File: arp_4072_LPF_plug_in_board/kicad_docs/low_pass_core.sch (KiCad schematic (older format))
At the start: 46 parts, among them Q1 BCM857DS, Q2 BCM857DS, Q3 BCM857DS, Q4 BCM857DS, Q5 BCM857DS, Q6 BCM857DS, U1 LM3900, U2 TL072, U3 TL072

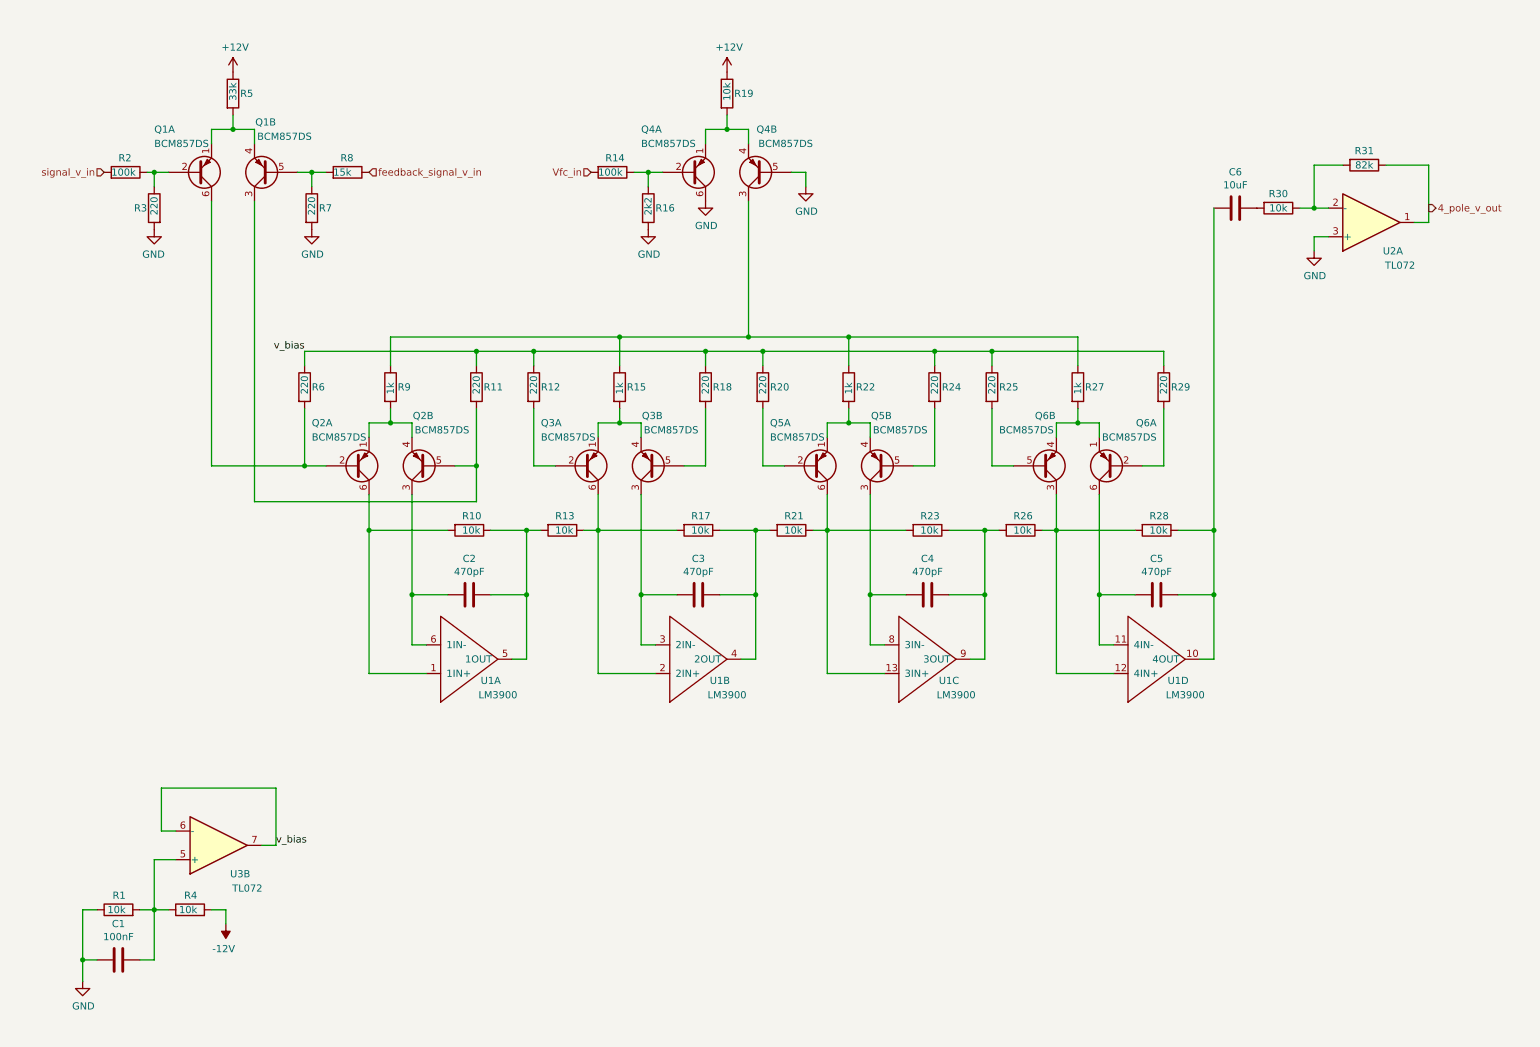
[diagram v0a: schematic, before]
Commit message: fix schemo and pcb problems
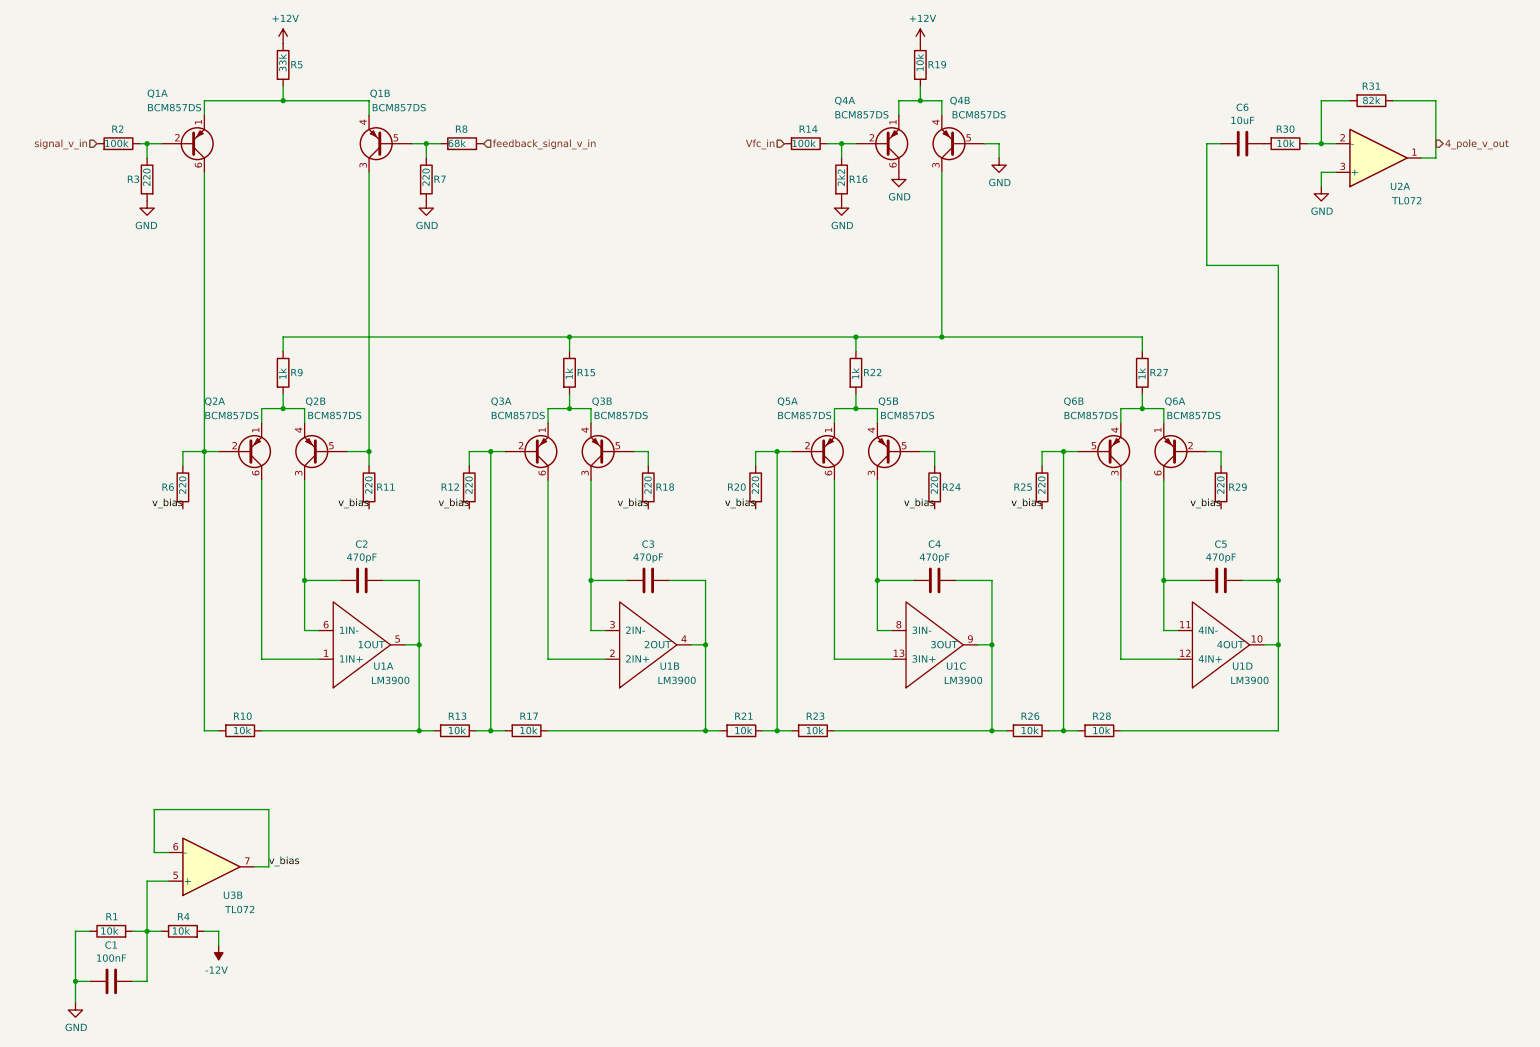
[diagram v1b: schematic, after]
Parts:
- R8: value 15k -> 68k
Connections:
- net v_bias: now also R11.2, R12.2, R18.2, R20.2, R24.2, R25.2, R29.2, R6.2; no longer R11.1, R12.1, R18.1, R20.1, R24.1, R25.1, R29.1, R6.1
- net at Q2.6 (C), U1.1 (1IN+): no longer R10.2
- net at Q1.6 (C), Q2.2 (B): now also R10.2, R6.1; no longer R6.2
- net at Q1.3 (C), Q2.5 (B): now also R11.1; no longer R11.2
- net at R13.1, R17.2: now also Q3.2 (B), R12.1; no longer Q3.6 (C), U1.2 (2IN+)
- net at Q3.5 (B): now also R18.1; no longer R18.2
- net at R21.1, R23.2: now also Q5.2 (B), R20.1; no longer Q5.6 (C), U1.13 (3IN+)
- net at Q5.5 (B): now also R24.1; no longer R24.2
- net at R26.1, R28.2: now also Q6.5 (B), R25.1; no longer Q6.3 (C), U1.12 (4IN+)
- net at Q6.2 (B): now also R29.1; no longer R29.2
- new net: Q3.6 (C), U1.2 (2IN+)
- new net: Q5.6 (C), U1.13 (3IN+)
- new net: Q6.3 (C), U1.12 (4IN+)
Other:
- moved on the sheet: C1, C2, C3, C4, C5, C6, Q1A, Q1B, Q2A, Q2B, Q3A, Q3B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
